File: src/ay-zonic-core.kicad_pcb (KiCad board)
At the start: 2 copper layers, 61 x 80.6 mm, 31 parts, among them J1 01x10, SW1 SW_DIP_x01, U1 AY-3-8912, U2 74HCT74, U3 74HCT08, U4 74HCT11, U5 74HCT02

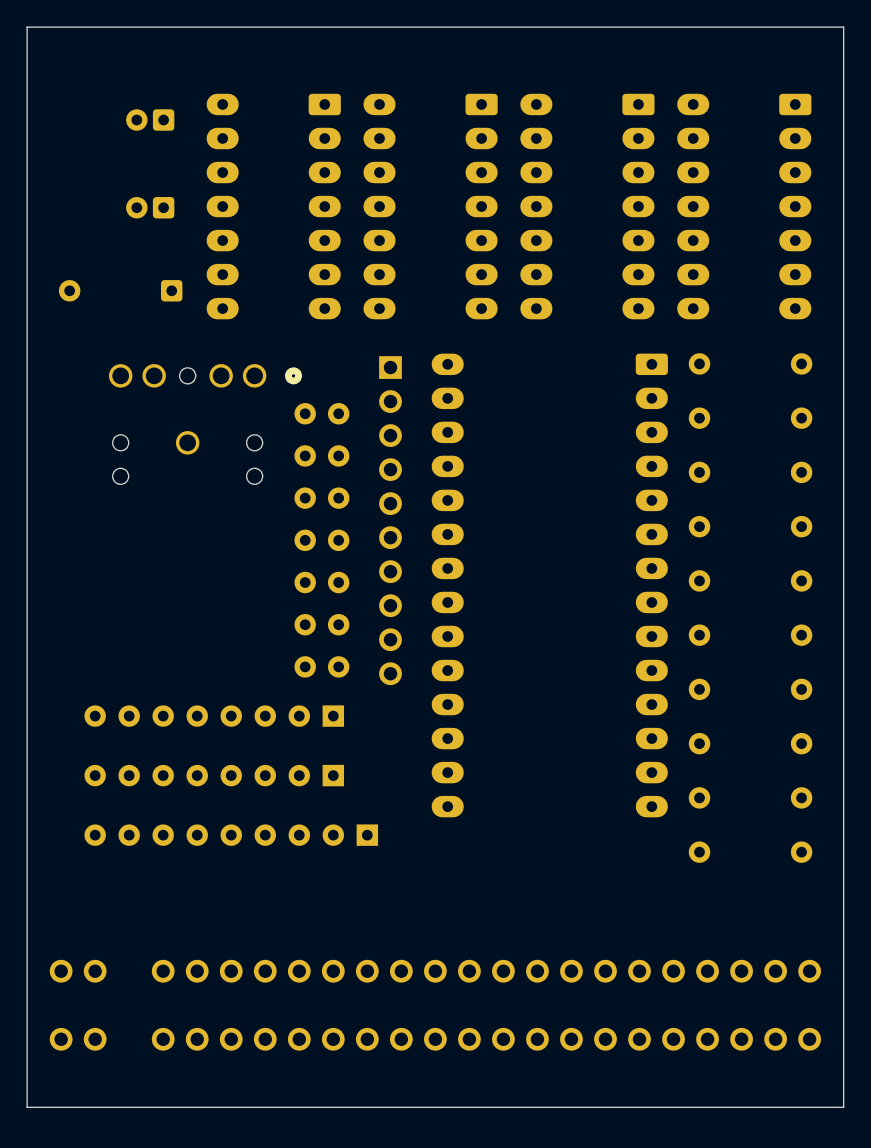
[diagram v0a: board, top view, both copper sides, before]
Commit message: Signed-off-by: jgratton72 <jon@grattons.co.uk>
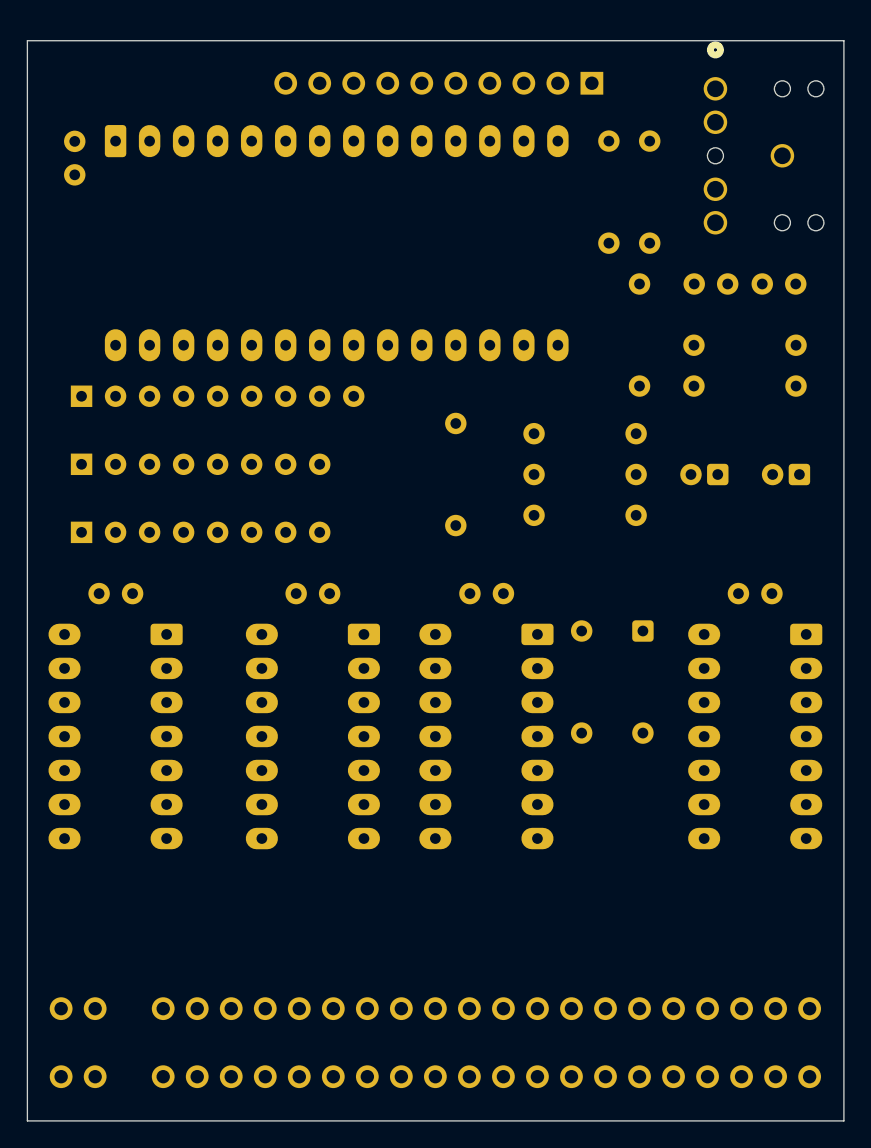
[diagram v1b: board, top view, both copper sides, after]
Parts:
- U2, U3, U4, U5: footprint Package_DIP:DIP-14_W7.62mm_Socket_LongPads -> Package_DIP:DIP-14_W7.62mm_LongPads
- moved U2 61.4 mm to (75.2, 93.0)
- moved C1 54.3 mm to (122.4, 81.0)
- moved U5 53.5 mm to (122.9, 93.0)
- moved C2 45.9 mm to (116.3, 81.0)
- moved U3 44.6 mm to (89.9, 93.0)
- moved SW1 43.4 mm to (110.7, 92.7), turned to -90 degrees
- moved U1 43.4 mm to (71.4, 56.1), turned to -90 degrees
- moved CO2 40.5 mm to (116.2, 52.2), turned to -90 degrees
- moved U4 39.8 mm to (102.9, 93.0)
- moved RN1 39.1 mm to (68.8, 75.2), turned to 0 degrees
- moved R8 38.7 mm to (114.6, 71.4), turned to 0 degrees
- moved C3 35.5 mm to (122.2, 66.8)
- moved R5 32.6 mm to (108.2, 63.8), turned to 90 degrees
- moved C4 31.8 mm to (117.1, 66.8)
- moved C5 31.2 mm to (68.3, 58.7), turned to 90 degrees
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- renumbered R11 to R8, R10 to R9
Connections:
- J1 pad 1: /IOA0 -> VCC
- J1 pad 2: /IOA1 -> /IOA0
- J1 pad 3: /IOA2 -> /IOA1
- J1 pad 4: /IOA3 -> /IOA2
- J1 pad 5: /IOA4 -> /IOA3
- J1 pad 6: /IOA5 -> /IOA4
- J1 pad 7: /IOA6 -> /IOA5
- J1 pad 8: /IOA7 -> /IOA6
- J1 pad 9: VCC -> /IOA7
